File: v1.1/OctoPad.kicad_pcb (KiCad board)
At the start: 2 copper layers, 286.6 x 138.1 mm, 22 parts, among them U1 ProMicro

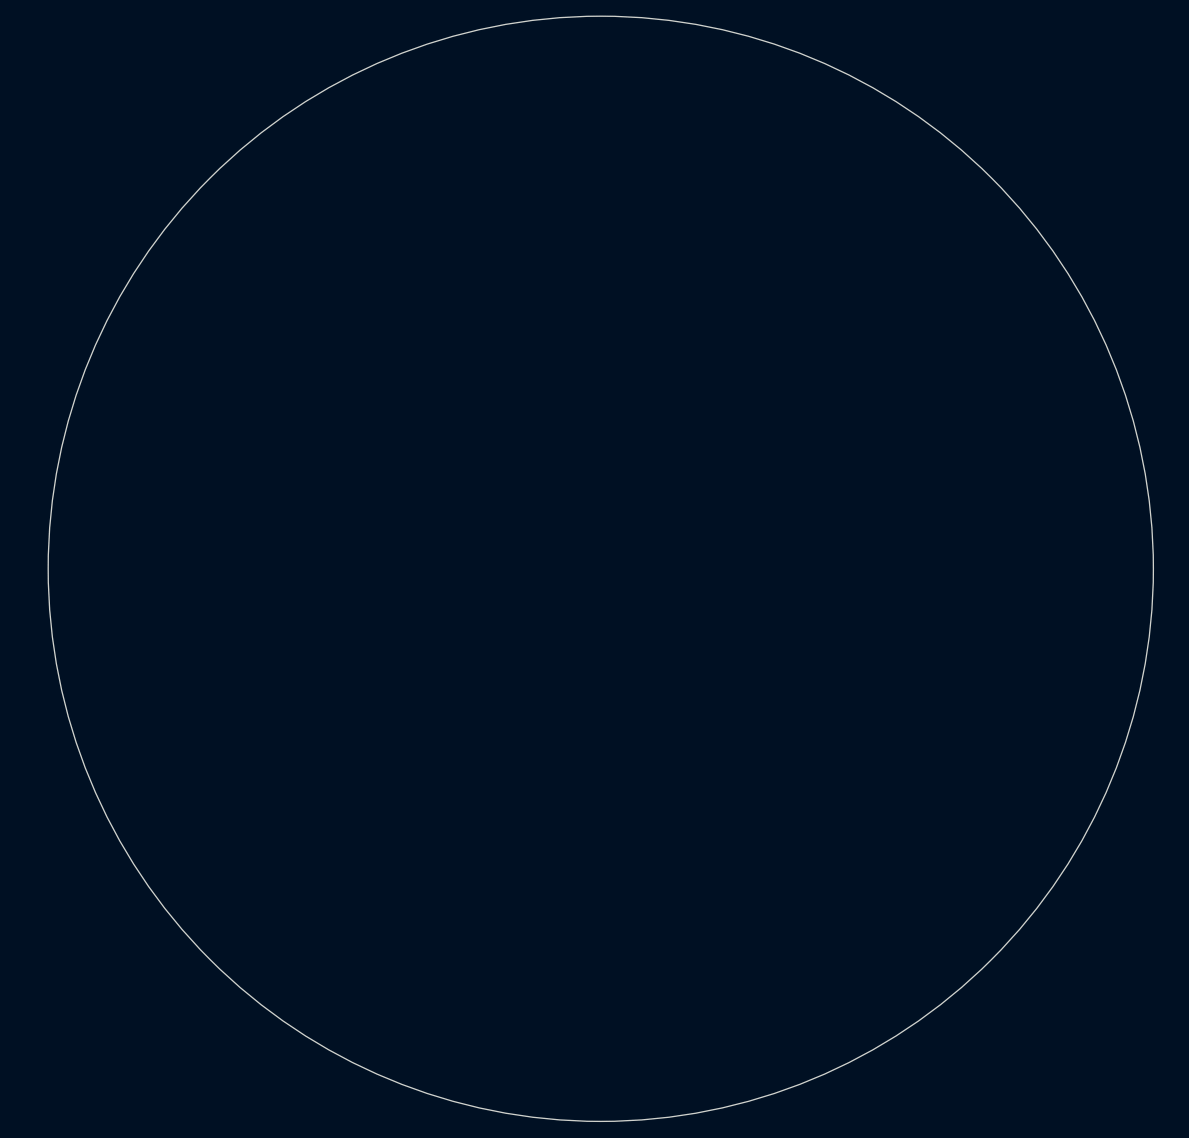
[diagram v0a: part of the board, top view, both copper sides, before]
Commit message: 4/6/20 v1
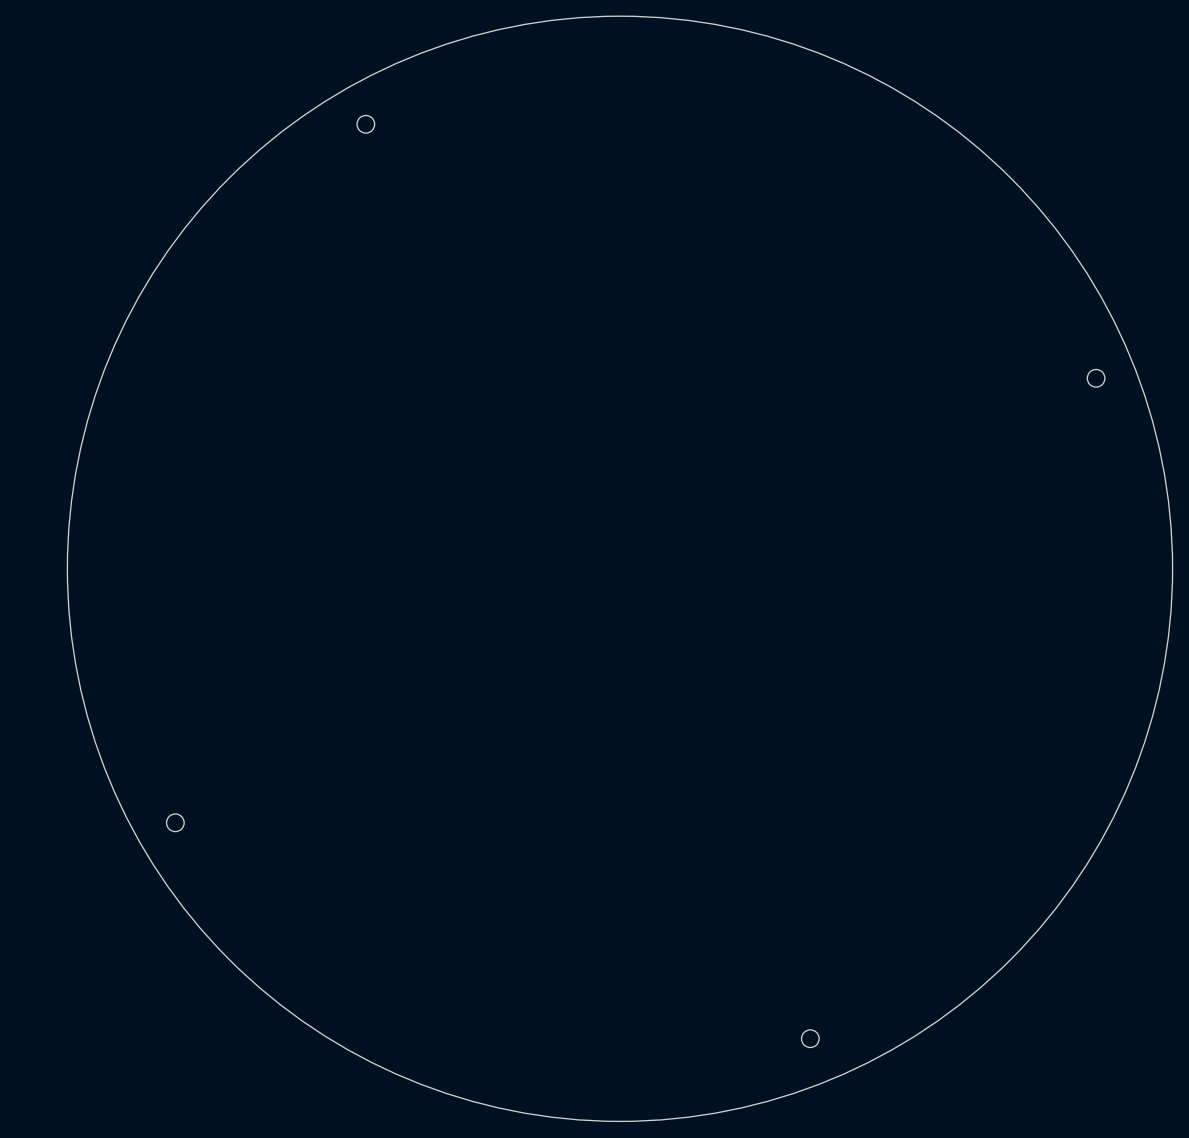
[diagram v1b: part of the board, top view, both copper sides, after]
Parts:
- added REF**: MountingHole_2.2mm_M2, MountingHole:MountingHole_2.2mm_M2, F.Cu at (334.2, 173.0)
- added REF**: MountingHole_2.2mm_M2, MountingHole:MountingHole_2.2mm_M2, F.Cu at (369.9, 90.5)
- added REF**: MountingHole_2.2mm_M2, MountingHole:MountingHole_2.2mm_M2, F.Cu at (278.6, 58.7)
- added REF**: MountingHole_2.2mm_M2, MountingHole:MountingHole_2.2mm_M2, F.Cu at (254.8, 146.1)
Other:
- board size 286.6 x 138.1 mm -> 289 x 138.1 mm
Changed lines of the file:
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@@
     (tracks 119)
     (zones 0)
-    (modules 22)
+    (modules 26)
     (nets 31)
   )
@@
   )
   (module MountingHole:MountingHole_2.2mm_M2 (layer F.Cu)
+    (at 334.16875 173.0375)
+    (descr "Mounting Hole 2.2mm, no annular, M2")
+    (tags "mounting hole 2.2mm no annular m2")
+    (attr virtual)
+    (fp_text reference REF** (at 0 -3.2) (layer F.SilkS) hide
+      (effects (font (size 1 1) (thickness 0.15)))
+    )
+    (fp_text value MountingHole_2.2mm_M2 (at 0 3.2) (layer F.Fab)
+      (effects (font (size 1 1) (thickness 0.15)))
+    )
+    (fp_circle (center 0 0) (end 2.45 0) (layer F.CrtYd) (width 0.05))
+    (fp_circle (center 0 0) (end 2.2 0) (layer Cmts.User) (width 0.15))
+    (fp_text user %R (at 0.3 0) (layer F.Fab)
+      (effects (font (size 1 1) (thickness 0.15)))
+    )
+    (pad 1 np_thru_hole circle (at 0 0) (size 2.2 2.2) (drill 2.2) (layers *.Cu *.Mask))
+  )
+  (module MountingHole:MountingHole_2.2mm_M2 (layer F.Cu)
+    (at 369.8875 90.4875)
+    (descr "Mounting Hole 2.2mm, no annular, M2")
+    (tags "mounting hole 2.2mm no annular m2")
+    (attr virtual)
+    (fp_text reference REF** (at 0 -3.2) (layer F.SilkS) hide
+      (effects (font (size 1 1) (thickness 0.15)))
+    )
+    (fp_text value MountingHole_2.2mm_M2 (at 0 3.2) (layer F.Fab)
+      (effects (font (size 1 1) (thickness 0.15)))
+    )
+    (fp_circle (center 0 0) (end 2.45 0) (layer F.CrtYd) (width 0.05))
+    (fp_circle (center 0 0) (end 2.2 0) (layer Cmts.User) (width 0.15))
+    (fp_text user %R (at 0.3 0) (layer F.Fab)
+      (effects (font (size 1 1) (thickness 0.15)))
+    )
+    (pad 1 np_thru_hole circle (at 0 0) (size 2.2 2.2) (drill 2.2) (layers *.Cu *.Mask))
+  )
+  (module MountingHole:MountingHole_2.2mm_M2 (layer F.Cu)
+    (at 278.60625 58.7375)
+    (descr "Mounting Hole 2.2mm, no annular, M2")
+    (tags "mounting hole 2.2mm no annular m2")
+    (attr virtual)
+    (fp_text reference REF** (at 0 -3.2) (layer F.SilkS) hide
+      (effects (font (size 1 1) (thickness 0.15)))
+    )
+    (fp_text value MountingHole_2.2mm_M2 (at 0 3.2) (layer F.Fab)
+      (effects (font (size 1 1) (thickness 0.15)))
+    )
+    (fp_circle (center 0 0) (end 2.45 0) (layer F.CrtYd) (width 0.05))
+    (fp_circle (center 0 0) (end 2.2 0) (layer Cmts.User) (width 0.15))
+    (fp_text user %R (at 0.3 0) (layer F.Fab)
+      (effects (font (size 1 1) (thickness 0.15)))
+    )
+    (pad 1 np_thru_hole circle (at 0 0) (size 2.2 2.2) (drill 2.2) (layers *.Cu *.Mask))
+  )
+  (module MountingHole:MountingHole_2.2mm_M2 (layer F.Cu)
+    (at 254.79375 146.05)
+    (descr "Mounting Hole 2.2mm, no annular, M2")
+    (tags "mounting hole 2.2mm no annular m2")
+    (attr virtual)
+    (fp_text reference REF** (at 0 -3.2) (layer F.SilkS) hide
+      (effects (font (size 1 1) (thickness 0.15)))
+    )
+    (fp_text value MountingHole_2.2mm_M2 (at 0 3.2) (layer F.Fab)
+      (effects (font (size 1 1) (thickness 0.15)))
+    )
+    (fp_text user %R (at 0.3 0) (layer F.Fab)
+      (effects (font (size 1 1) (thickness 0.15)))
+    )
+    (fp_circle (center 0 0) (end 2.2 0) (layer Cmts.User) (width 0.15))
+    (fp_circle (center 0 0) (end 2.45 0) (layer F.CrtYd) (width 0.05))
+    (pad 1 np_thru_hole circle (at 0 0) (size 2.2 2.2) (drill 2.2) (layers *.Cu *.Mask))
+  )
+  (module MountingHole:MountingHole_2.2mm_M2 (layer F.Cu)
     (at 183.35625 173.0375)
     (descr "Mounting Hole 2.2mm, no annular, M2")
@@
   )
   (gr_line (start 94.45625 100.80625) (end 98.425 102.39375) (layer F.SilkS) (width 0.12))
-  (gr_circle (center 307.975 114.3) (end 238.91875 112.7125) (layer Edge.Cuts) (width 0.05))
+  (gr_circle (center 310.374494 114.3) (end 241.318244 112.7125) (layer Edge.Cuts) (width 0.05))
   (gr_text rev1.1 (at 159.54375 135.73125) (layer F.SilkS)
     (effects (font (size 1.5 1.5) (thickness 0.3)))
